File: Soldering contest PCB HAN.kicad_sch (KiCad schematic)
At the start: 13 parts, among them J1 Screw_Terminal_01x02, Q1 2N3904, Q2 2N3904

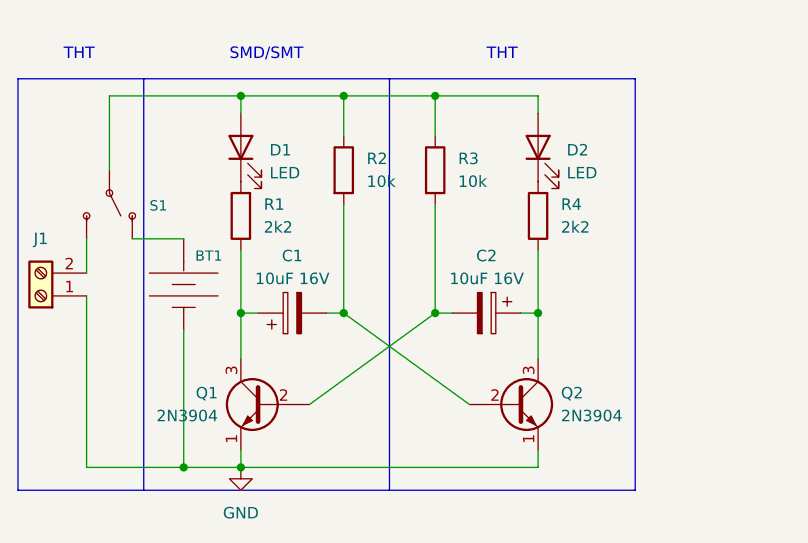
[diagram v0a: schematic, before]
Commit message: improved wiring and connected everything
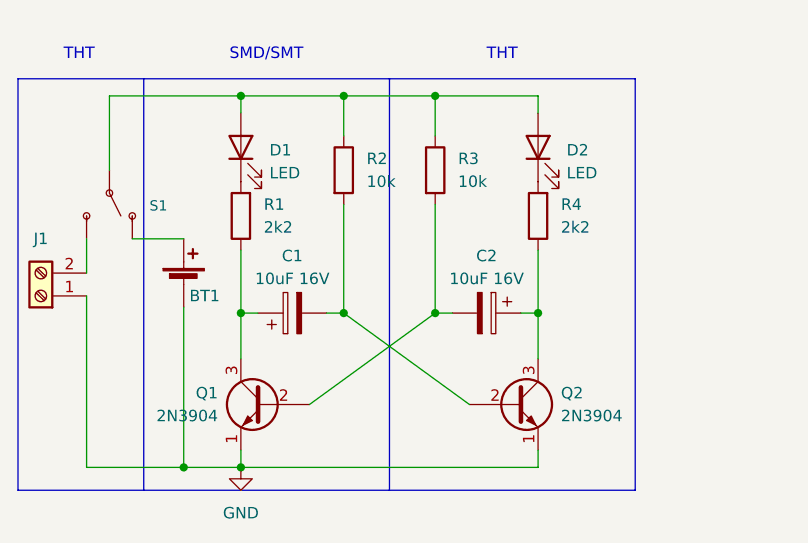
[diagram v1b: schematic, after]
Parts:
- removed BT1: BATTERY-6.8MM_SMD, Battery:BatteryHolder_Keystone_3002_1x2032, symbol SparkFun-Batteries:BATTERY-6.8MM_SMD
- added BT1: Battery_Cell, Battery:BatteryHolder_Keystone_3002_1x2032, symbol Device:Battery_Cell
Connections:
- net GND: now also BT1.2 (-)
- net at S1.1 (O): now also BT1.1 (+)
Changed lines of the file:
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@@
     (stroke (width 0) (type default) (color 0 0 0 0))
   )
-  (wire (pts (xy 71.755 74.93) (xy 71.755 90.17))
+  (wire (pts (xy 71.755 72.39) (xy 71.755 90.17))
     (stroke (width 0) (type default) (color 0 0 0 0))
   )
@@
     (pin "2")
   )
-  (symbol (lib_id "SparkFun-Batteries:BATTERY-6.8MM_SMD") (at 71.755 69.85 270) (unit 1)
-    (in_bom yes) (on_board yes)
-    (property "Reference" "BT1" (id 0) (at 73.025 66.675 90)
-      (effects (font (size 1.143 1.143)) (justify left))
-    )
-    (property "Value" "BATTERY-6.8MM_SMD" (id 1) (at 76.835 69.85 90)
-      (effects (font (size 1.143 1.143)) (justify left) hide)
-    )
-    (property "Footprint" "Battery:BatteryHolder_Keystone_3002_1x2032" (id 2) (at 78.105 69.85 0)
-      (effects (font (size 0.508 0.508)) hide)
-    )
-    (property "Datasheet" "" (id 3) (at 71.755 69.85 0)
-      (effects (font (size 1.27 1.27)) hide)
-    )
-    (property "Field4" "BATT-13734" (id 4) (at 76.835 73.025 90)
-      (effects (font (size 1.524 1.524)) (justify left) hide)
-    )
-    (property "Purpose" "C2032" (id 5) (at 85.725 68.58 90)
-      (effects (font (size 1.27 1.27)) hide)
-    )
-    (pin "+")
-    (pin "-")
-  )
   (symbol (lib_id "Device:C_Polarized") (at 83.82 73.025 90) (unit 1)
     (in_bom yes) (on_board yes)
@@
     (pin "1")
   )
+  (symbol (lib_id "Device:Battery_Cell") (at 71.755 69.85 0) (unit 1)
+    (in_bom yes) (on_board yes)
+    (property "Reference" "BT1" (id 0) (at 72.39 71.12 0)
+      (effects (font (size 1.27 1.27)) (justify left))
+    )
+    (property "Value" "Battery_Cell" (id 1) (at 74.93 69.0879 0)
+      (effects (font (size 1.27 1.27)) (justify left) hide)
+    )
+    (property "Footprint" "Battery:BatteryHolder_Keystone_3002_1x2032" (id 2) (at 71.755 68.326 90)
+      (effects (font (size 1.27 1.27)) hide)
+    )
+    (property "Datasheet" "~" (id 3) (at 71.755 68.326 90)
+      (effects (font (size 1.27 1.27)) hide)
+    )
+    (pin "1")
+    (pin "2")
+  )
   (sheet_instances
     (path "/" (page "1"))
@@
       (reference "#PWR01") (unit 1) (value "GND") (footprint "")
     )
-    (path "/44a5ce8e-2c11-4619-8ce9-b752075d2088"
-      (reference "BT1") (unit 1) (value "BATTERY-6.8MM_SMD") (footprint "Battery:BatteryHolder_Keystone_3002_1x2032")
+    (path "/ff5ddebd-fa0b-425a-8582-07d48577659b"
+      (reference "BT1") (unit 1) (value "Battery_Cell") (footprint "Battery:BatteryHolder_Keystone_3002_1x2032")
     )
     (path "/5c87c882-b6f1-48af-94eb-8b3a9c0bcf0b"

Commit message: archived 3d models
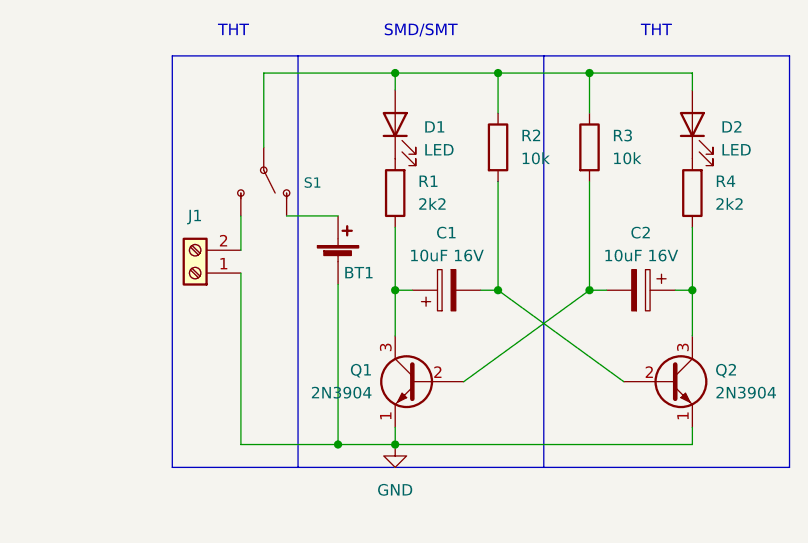
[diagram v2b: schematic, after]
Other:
- moved on the sheet: BT1, C1, C2, D1, D2, J1, Q1, Q2, R1, R2, R3, R4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
